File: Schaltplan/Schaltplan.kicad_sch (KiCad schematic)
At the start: 15 parts, among them P1 USB_C_Plug_USB2.0, P2 USB_C_Plug_USB2.0, P3 USB_C_Plug_USB2.0, U1 ACS712xLCTR-05B, U2 LM2596S, U3 DS18B20, U4 DS18B20, U5 LM2596S, U6 DS3502, U7 DS3502, U8 LM2596S

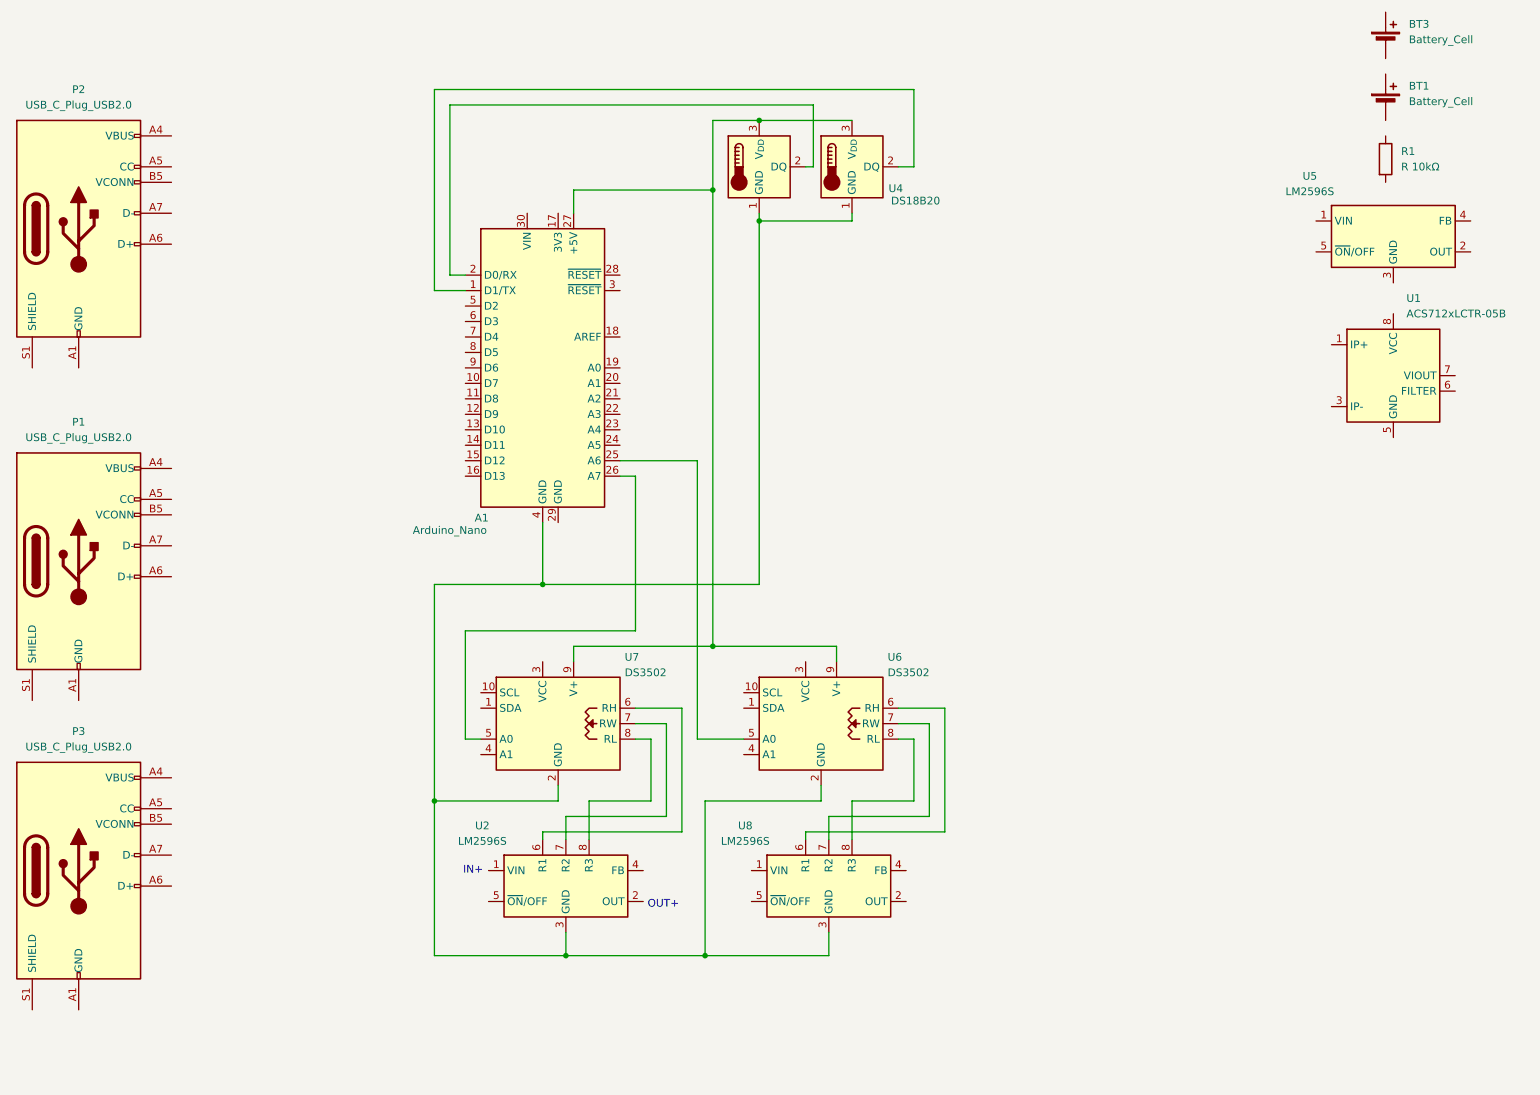
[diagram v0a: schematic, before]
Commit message: Weird Stuff hapened
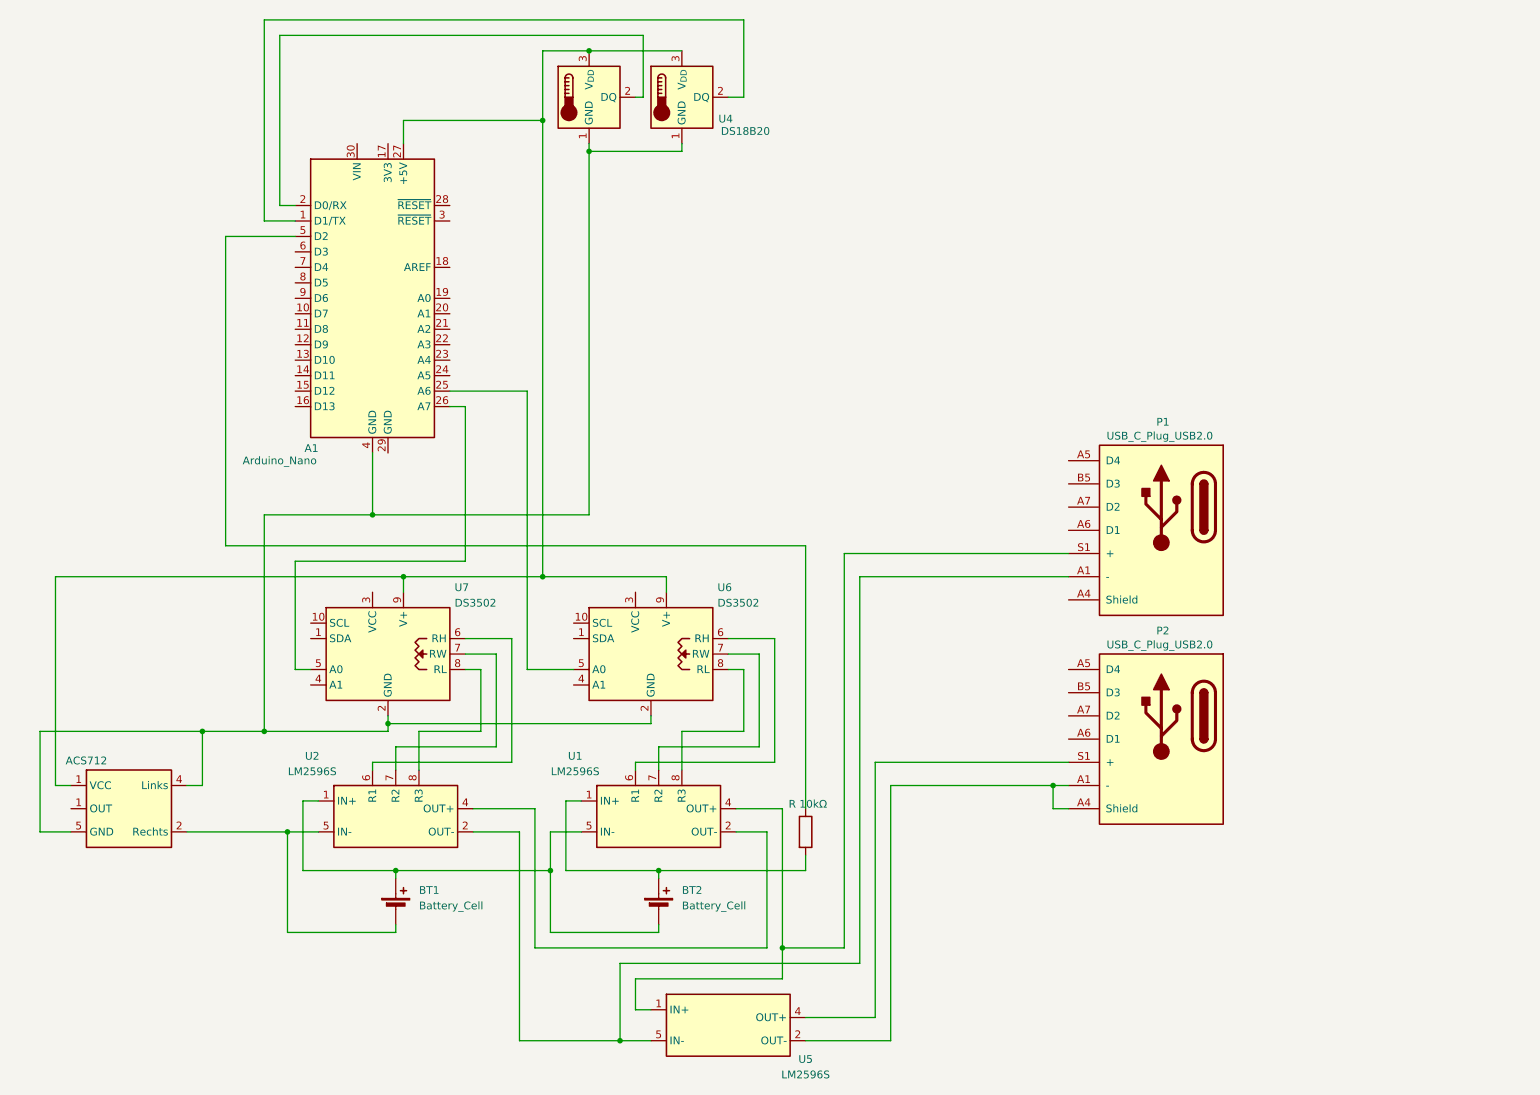
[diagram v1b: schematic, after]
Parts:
- removed BT3: Battery_Cell, symbol Device:Battery_Cell
- removed P3: USB_C_Plug_USB2.0, symbol Connector:USB_C_Plug_USB2.0
- removed U1: ACS712xLCTR-05B, Package_SO:SOIC-8_3.9x4.9mm_P1.27mm, symbol Sensor_Current:ACS712xLCTR-05B
- added BT2: Battery_Cell, symbol Device:Battery_Cell
- added U1: LM2596S, Package_TO_SOT_SMD:TO-263-5_TabPin3, symbol Regulator_Switching:LM2596S-5
- U8: value LM2596S -> ACS712
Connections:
- net at U8.2 (Rechts): now also BT1.2 (-), U2.5 (IN-)
- net at A1.4 (GND), U3.1 (GND), U4.1 (GND)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: now also U8.4 (Links), U8.5 (GND); no longer U2.3 (GND), U8.3 (GND)
- net at U6.6 (RH): now also U1.6 (R1); no longer U8.6 (R1)
- net at U6.7 (RW): now also U1.7 (R2); no longer U8.7 (R2)
- net at U6.8 (RL): now also U1.8 (R3); no longer U8.8 (R3)
- net at BT1.1 (+): now also U2.1 (IN+), BT2.2 (-), U1.5 (IN-)
- net at A1.27 (+5V), U3.3 (V_{DD}), U4.3 (V_{DD})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: now also U8.1 (OUT)
- net at U5.1 (IN+): now also P1.S1 (+), U1.4 (OUT+)
- net at U5.2 (OUT-): now also P2.A1 (-), P2.A4 (Shield)
- net at U5.4 (OUT+): now also P2.S1 (+)
- net at U5.5 (IN-): now also P1.A1 (-), U2.2 (OUT-)
- net at R1.1: now also A1.5 (D2)
- net at R1.2: now also BT2.1 (+), U1.1 (IN+)
- net at U2.4 (OUT+): now also U1.2 (OUT-)
- net at P1.A12 (GND), P1.B1 (GND), P1.B12 (GND): no longer P1.A1 (GND)
- net at P1.A9 (VBUS), P1.B4 (VBUS), P1.B9 (VBUS): no longer P1.A4 (VBUS)
- net at P2.A12 (GND), P2.B1 (GND), P2.B12 (GND): no longer P2.A1 (GND)
- net at P2.A9 (VBUS), P2.B4 (VBUS), P2.B9 (VBUS): no longer P2.A4 (VBUS)
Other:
- note removed: "IN+"
- note removed: "OUT+"
- moved on the sheet: A1, BT1, U4, U6, U7
